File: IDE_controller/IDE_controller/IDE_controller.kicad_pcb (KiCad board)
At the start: 2 copper layers, 66 parts, among them CON2 Conn_02x17_Odd_Even, J1 Bus_ISA_16bit_narrow, J10 Conn_01x02, J2 DA15_Socket, U11 C820101A, U12 74LS245, U13 74LS245, U14 74LS245, U2 74LS125, U4 W86C450, U5 W86C450, U8 UM82C11

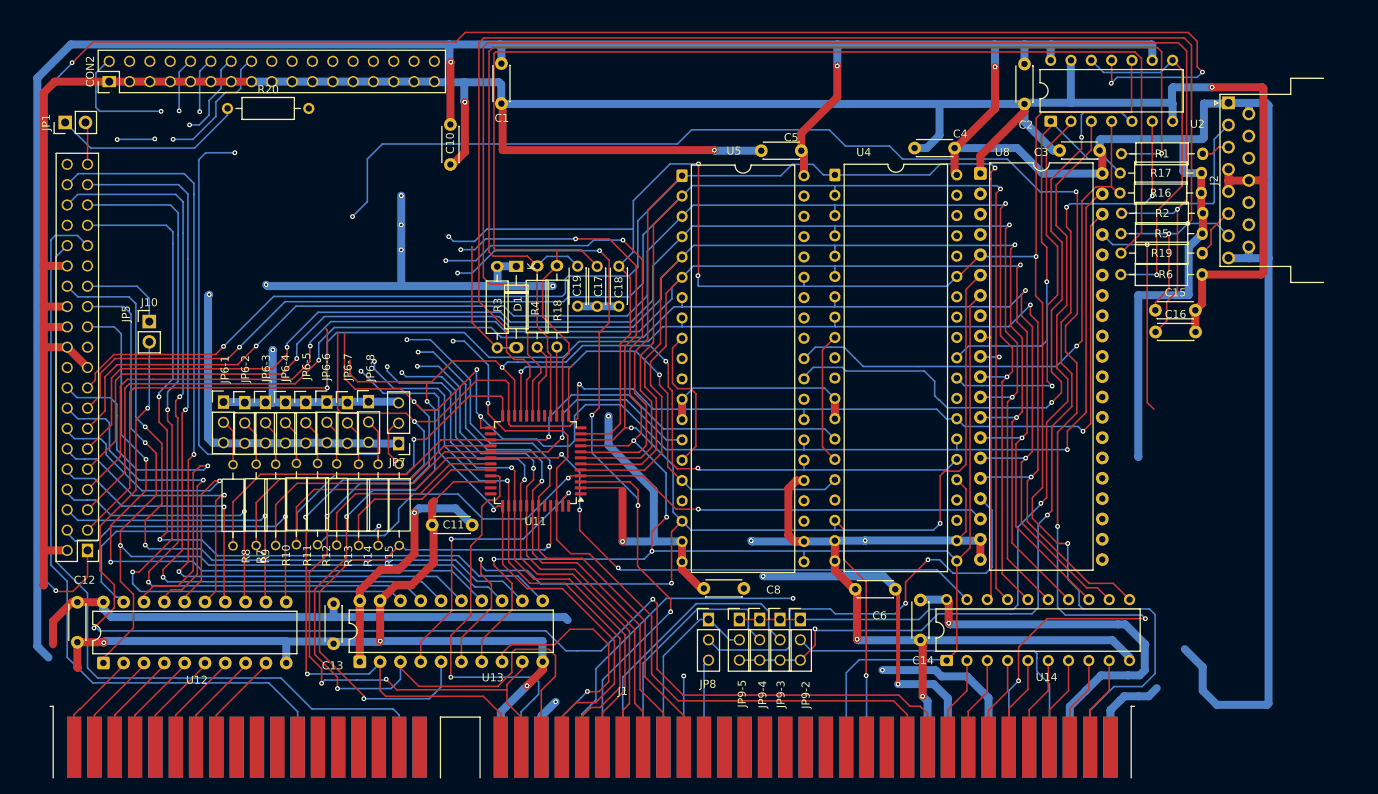
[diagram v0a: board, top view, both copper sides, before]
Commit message: IDE controller update
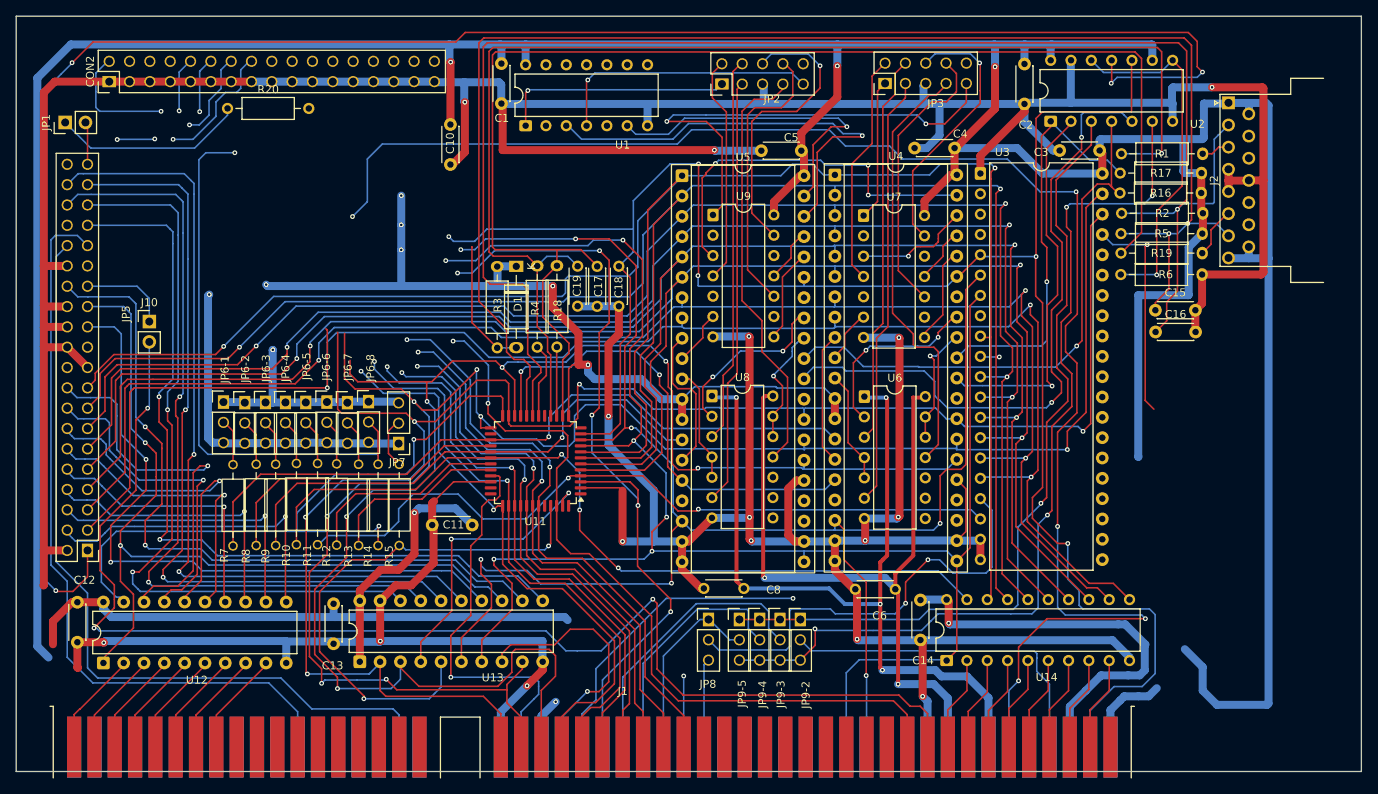
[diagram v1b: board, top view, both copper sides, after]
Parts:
- added JP2: Conn_02x05_Odd_Even, Connector_PinHeader_2.54mm:PinHeader_2x05_P2.54mm_Vertical, F.Cu at (159.1, 52.9)
- added JP3: Conn_02x05_Odd_Even, Connector_PinHeader_2.54mm:PinHeader_2x05_P2.54mm_Vertical, F.Cu at (179.5, 52.8)
- added U1: SN75189, Package_DIP:DIP-14_W7.62mm, F.Cu at (134.6, 58.1)
- added U6: 74HC00, Package_DIP:DIP-14_W7.62mm, F.Cu at (176.9, 91.9)
- added U7: SN75189, Package_DIP:DIP-14_W7.62mm, F.Cu at (176.8, 69.3)
- added U8: 74HC00, Package_DIP:DIP-14_W7.62mm, F.Cu at (157.9, 91.8)
- added U9: SN75189, Package_DIP:DIP-14_W7.62mm, F.Cu at (158.0, 69.2)
- J2: value DA15_Socket -> GAMEPORT
- U4, U5: footprint Package_DIP:DIP-40_W15.24mm -> Package_DIP:DIP-40_W15.24mm_Socket
- renumbered U8 to U3
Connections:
- net /GND renamed GND
- net /IRQ2 renamed IRQ2
- net /IRQ3 renamed IRQ3
- net /IRQ4 renamed IRQ4
- net /IRQ5 renamed IRQ5
- net /U8_CS renamed /~{PARALLEL_CS}
- net /jp9-2 renamed /Serial/jp9-2
- net /jp9-3 renamed /Serial/jp9-3
- net /u11-14 renamed Net-(C17-Pad2)
- net /u11-15 renamed Net-(R18-Pad1)
- net /u11-16 renamed Net-(C19-Pad2)
- net /u11-18 renamed Net-(R4-Pad1)
- net /u11-21 renamed /UART_CLK
- net /u2-5 renamed Net-(U5-INTR)
- net /u4-15 renamed Net-(U4-RCLK)
- net /u4-30 renamed Net-(U4-INTR)
- net /u4-31 renamed Net-(U4-~{OUT2})
- net /u5-15 renamed Net-(U5-RCLK)
- net /u5-31 renamed Net-(U5-~{OUT2})
- C1 pad 2: /+5V -> +5V
- C10 pad 2: /+5V -> +5V
- C11 pad 2: /+5V -> +5V
- C12 pad 2: /+5V -> +5V
- C13 pad 2: /+5V -> +5V
- C14 pad 2: /+5V -> +5V
- C2 pad 2: /+5V -> +5V
- C3 pad 2: /+5V -> +5V
- C4 pad 2: /+5V -> +5V
- C5 pad 2: /+5V -> +5V
- C8 pad 2: /+5V -> /-12V
- D1 pad 1: /+5V -> +5V
- J1 pad 29: /+5V -> +5V
- J1 pad 3: /+5V -> +5V
- J1 pad 78: /+5V -> +5V
- J2 pad 1: /+5V -> +5V
- J2 pad 15: /+5V -> +5V
- J2 pad 8: /+5V -> +5V
- J2 pad 9: /+5V -> +5V
- JP6-1 pad 1: /+5V -> +5V
- JP6-2 pad 1: /+5V -> +5V
- JP6-3 pad 1: /+5V -> +5V
- JP6-4 pad 1: /+5V -> +5V
- JP6-5 pad 1: /+5V -> +5V
- JP6-6 pad 1: /+5V -> +5V
- JP6-7 pad 1: /+5V -> +5V
- JP6-8 pad 1: /+5V -> +5V
- JP7 pad 3: /+5V -> +5V
- R16 pad 2: /+5V -> +5V
- R17 pad 2: /+5V -> +5V
- R2 pad 2: /+5V -> +5V
- R20 pad 2: /+5V -> +5V
- R3 pad 2: /+5V -> +5V
- R5 pad 2: /+5V -> +5V
- U11 pad 13: /+5V -> +5V
- U11 pad 35: /+5V -> +5V
- U12 pad 20: /+5V -> +5V
- U13 pad 1: /+5V -> +5V
- U13 pad 20: /+5V -> +5V
- U14 pad 20: /+5V -> +5V
- U2 pad 14: /+5V -> +5V
- U2 pad 9: /+5V -> +5V
- U3 pad 40: /+5V -> +5V
- U4 pad 10: unconnected-(U4-SIN-Pad10) -> Net-(U4-SIN)
- U4 pad 11: unconnected-(U4-SOUT-Pad11) -> Net-(U4-SOUT)
- U4 pad 12: /+5V -> +5V
- U4 pad 13: /+5V -> +5V
- U4 pad 32: unconnected-(U4-~{RTS}-Pad32) -> Net-(U4-~{RTS})
- U4 pad 33: unconnected-(U4-~{DTR}-Pad33) -> Net-(U4-~{DTR})
- U4 pad 36: unconnected-(U4-~{CTS}-Pad36) -> Net-(U4-~{CTS})
- U4 pad 37: unconnected-(U4-~{DSR}-Pad37) -> Net-(U4-~{DSR})
- U4 pad 38: unconnected-(U4-~{DCO}-Pad38) -> Net-(U4-~{DCD})
- U4 pad 39: unconnected-(U4-~{RI}-Pad39) -> Net-(U4-~{RI})
- U4 pad 40: /+5V -> +5V
- U5 pad 10: unconnected-(U5-SIN-Pad10) -> Net-(U5-SIN)
- U5 pad 11: unconnected-(U5-SOUT-Pad11) -> Net-(U5-SOUT)
- U5 pad 12: /+5V -> +5V
- U5 pad 13: /+5V -> +5V
- U5 pad 32: unconnected-(U5-~{RTS}-Pad32) -> Net-(U5-~{RTS})
- U5 pad 33: unconnected-(U5-~{DTR}-Pad33) -> Net-(U5-~{DTR})
- U5 pad 36: unconnected-(U5-~{CTS}-Pad36) -> Net-(U5-~{CTS})
- U5 pad 37: unconnected-(U5-~{DSR}-Pad37) -> Net-(U5-~{DSR})
- U5 pad 38: unconnected-(U5-~{DCO}-Pad38) -> Net-(U5-~{DCD})
- U5 pad 39: unconnected-(U5-~{RI}-Pad39) -> Net-(U5-~{RI})
- U5 pad 40: /+5V -> +5V
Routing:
- net +5V: track 0.00 -> 785.9 mm, vias 0 -> 13
- net /+5V: track 742.0 -> 0.00 mm, vias 12 -> 0
- net GND: track 693.0 -> 789.1 mm, vias 13 -> 17
- net /-12V: track 20.8 -> 103.5 mm, vias 1 -> 4
- net /Serial/RI_1: track 0.00 -> 59.6 mm, vias 0 -> 2
- net Net-(U5-~{DCD}): track 0.00 -> 54.4 mm, vias 0 -> 1
- net /Serial/RTS_1: track 0.00 -> 54.4 mm
- net /Serial/TXD_1: track 0.00 -> 54.0 mm
- net /Serial/TXD_2: track 0.00 -> 53.3 mm
- net /Serial/RTS_2: track 0.00 -> 53.2 mm
- net /+12V: track 42.3 -> 92.4 mm
- net /Serial/DTR_1: track 0.00 -> 48.9 mm
- net /Serial/DTR_2: track 0.00 -> 48.3 mm
- net Net-(U4-~{RI}): track 0.00 -> 47.2 mm, vias 0 -> 3
- net Net-(U5-~{RI}): track 0.00 -> 41.2 mm, vias 0 -> 1
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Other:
- board outline added: 168.1 x 94.4 mm
